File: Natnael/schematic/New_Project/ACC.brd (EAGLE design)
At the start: 100 x 100 mm, 15 parts, among them J4 1935161

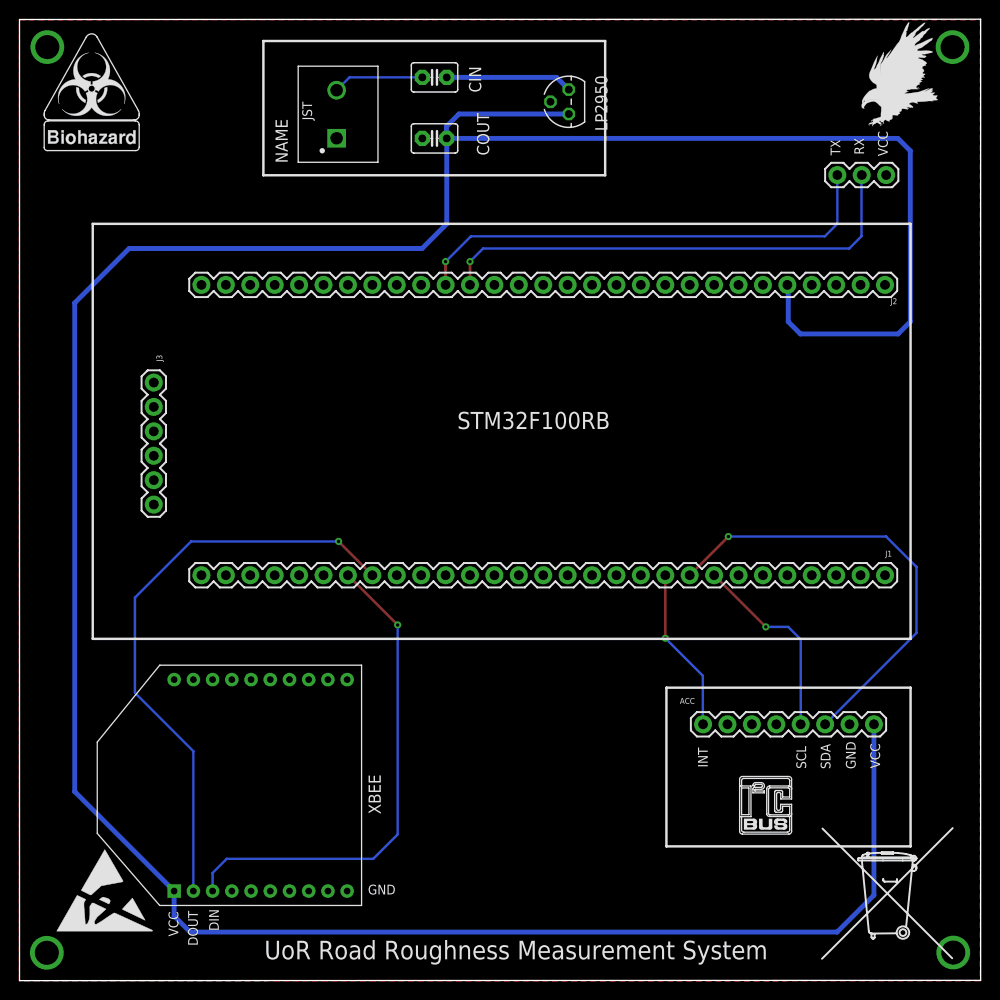
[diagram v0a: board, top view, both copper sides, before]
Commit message: pcb gerber files generated
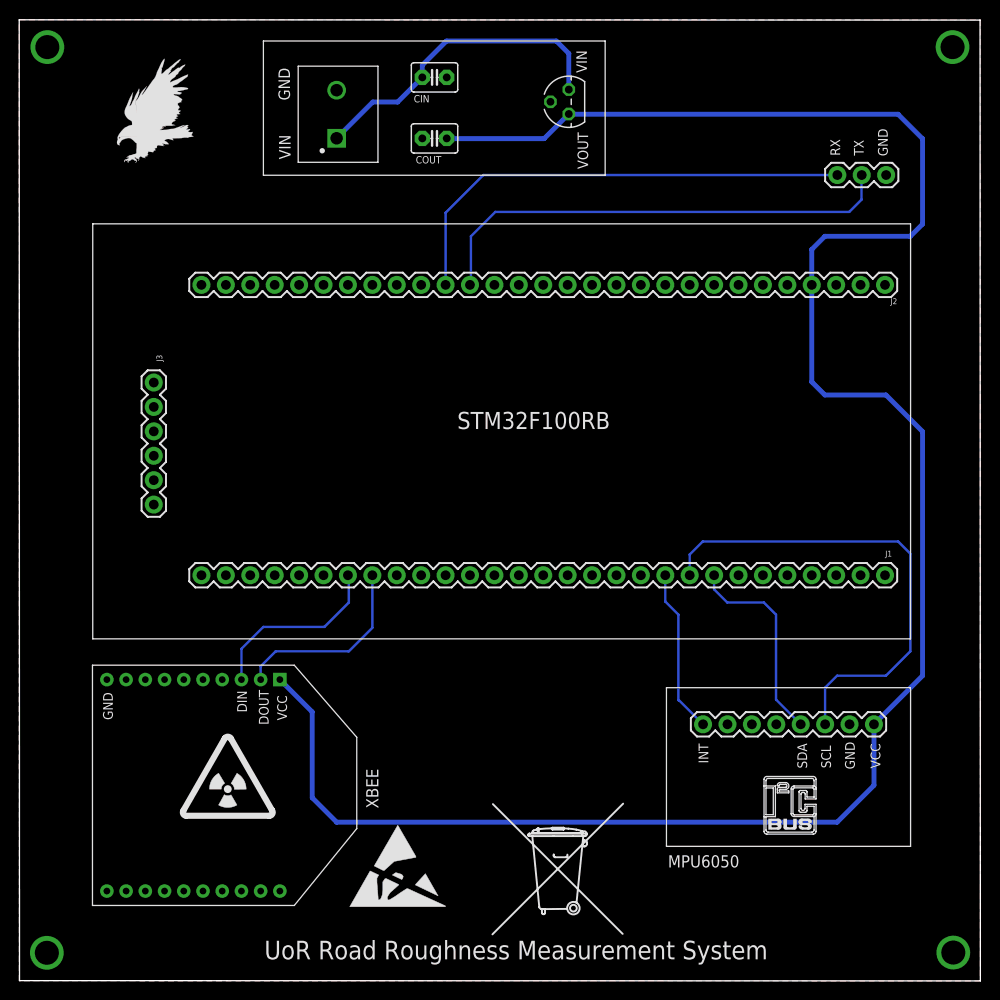
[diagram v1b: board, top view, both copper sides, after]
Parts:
- removed U$1: (no value), logo:BIOHAZARD_10.00
- added U$6: (no value), logo:RADIOACTIVE_10.00
- CIN: value (none) -> 1uF
- COUT: value (none) -> 2.2uF
- moved U$2 77.6 mm to (10.2, 85.1)
- moved U$4 34.4 mm to (55.9, 8.89)
- moved U$3 30.6 mm to (34.3, 7.62)
- moved U$5 2.54 mm to (77.5, 15.2)
- turned XBEE to 270 degrees
- renumbered ACC to MPU6050
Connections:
- removed net 3V3S: J2.4
- removed net N$1: CIN.1, J4.2
- removed net N$2: CIN.2, LP2950.3
- new net VBAT: J2.5
- new net VIN: CIN.1, J4.1, LP2950.3
- net 3V3: now also J2.4; no longer J2.5
- net GND: now also CIN.2, J4.2; no longer J4.1
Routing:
- net 3V3: track 310.6 -> 214.3 mm, vias 1 -> 0
- net PA10: track 61.6 -> 20.1 mm, vias 1 -> 0
- net VIN: track 0.00 -> 33.4 mm
- net PA9: track 51.9 -> 19.2 mm, vias 1 -> 0
- net N$2: track 13.2 -> 0.00 mm
- net N$1: track 9.47 -> 0.00 mm
- net PB6: track 46.9 -> 50.6 mm, vias 1 -> 0
- net PB7: track 20.6 -> 21.5 mm, vias 1 -> 0
- net PA2: track 50.6 -> 49.9 mm, vias 1 -> 0
- net PB5: track 17.1 -> 17.2 mm, vias 1 -> 0
- net PA3: vias 1 -> 0
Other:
- board text added: "VIN"
- board text added: "VOUT"
- board text removed: "JST"
